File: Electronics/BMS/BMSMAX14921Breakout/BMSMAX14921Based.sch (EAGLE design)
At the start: 66 parts, among them IC1 MAX14921, J1 CONNECTOR_9PIN, J4 CONNECTOR_9PIN, J5 CONNECTOR_8PIN, J6 CONNECTOR_9PIN

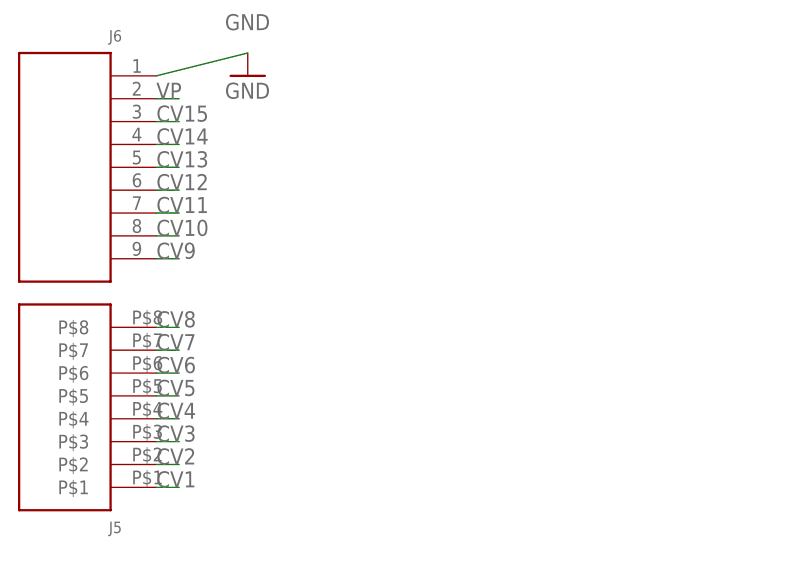
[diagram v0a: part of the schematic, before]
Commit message: pcb spacer and breakoutoard over
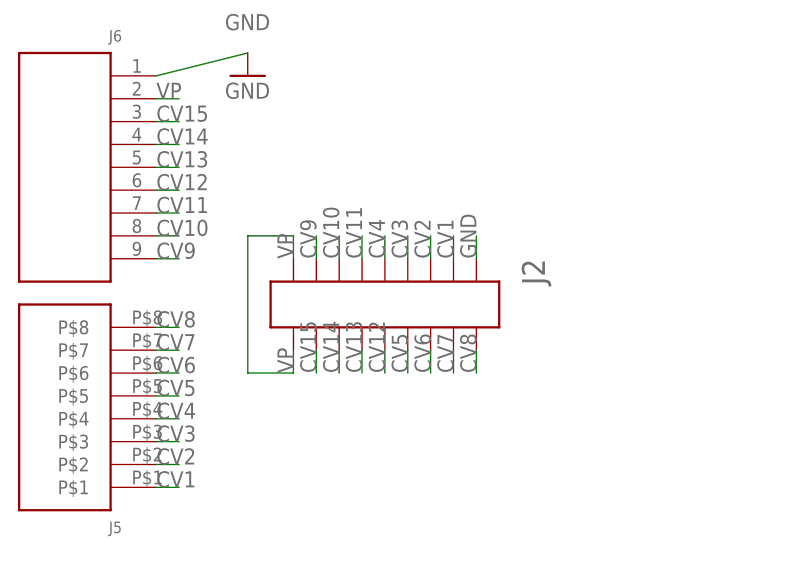
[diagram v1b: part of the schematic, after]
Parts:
- added J2: CONNECTORJST2X9_2MM, MarkIIEaglelbr:CONNECTORJST2X9_2MM
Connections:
- net CV1: now also J2.P$2
- net CV10: now also J2.P$7
- net CV11: now also J2.P$6
- net CV12: now also J2.P$14
- net CV13: now also J2.P$13
- net CV14: now also J2.P$12
- net CV15: now also J2.P$11
- net CV2: now also J2.P$3
- net CV3: now also J2.P$4
- net CV4: now also J2.P$5
- net CV5: now also J2.P$15
- net CV6: now also J2.P$16
- net CV7: now also J2.P$17
- net CV8: now also J2.P$18
- net CV9: now also J2.P$8
- net GND: now also J2.P$1
- net VP: now also J2.P$10, J2.P$9
